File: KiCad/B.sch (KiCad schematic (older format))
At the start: 6 parts

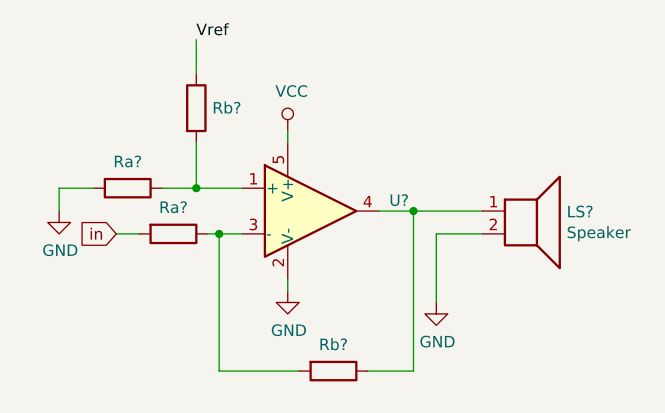
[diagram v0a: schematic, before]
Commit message: update schematics and libraries
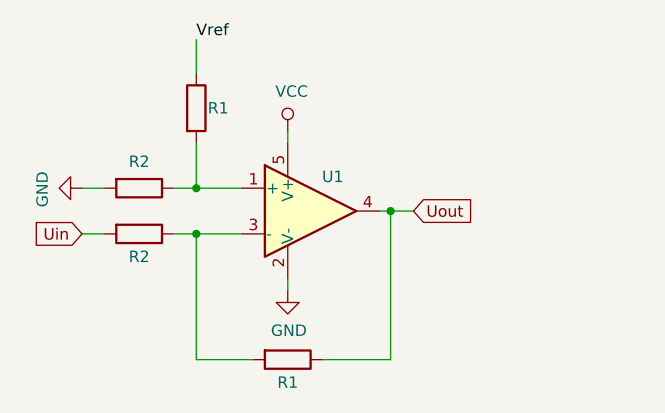
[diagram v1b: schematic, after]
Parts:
- removed LS?: Speaker, symbol Device:Speaker
- Ra3, Ra4: renamed from Ra?; value R -> R2
- Rb3, Rb4: renamed from Rb?; value R -> R1
- U2: renamed from U?; value LM321 -> U1
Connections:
- net Uout: now reaches Rb4.1, U2.4
- net in renamed Uin
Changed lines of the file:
@@
 $EndDescr
 $Comp
-L Amplifier_Operational:LM321 U?
+L Amplifier_Operational:LM321 U2
 U 1 1 617891E9
 P 5750 3750
-F 0 "U?" H 6094 3796 50  0000 L CNN
-F 1 "LM321" H 6094 3705 50  0001 L CNN
+F 0 "U2" H 6094 3796 50  0001 L CNN
+F 1 "U1" H 5800 3900 50  0000 L CNN
 F 2 "Package_TO_SOT_SMD:SOT-23-5" H 5750 3750 50  0001 C CNN
 F 3 "http://www.ti.com/lit/ds/symlink/lm321.pdf" H 5750 3750 50  0001 C CNN
@@
 	1    0    0    -1
 $EndComp
-$Comp
-L Device:Speaker LS?
-U 1 1 617891EF
-P 6700 3750
-F 0 "LS?" H 6870 3746 50  0000 L CNN
-F 1 "Speaker" H 6870 3655 50  0000 L CNN
-F 2 "" H 6700 3550 50  0001 C CNN
-F 3 "~" H 6690 3700 50  0001 C CNN
-	1    6700 3750
-	1    0    0    -1
-$EndComp
 Wire Wire Line
-	6500 3850 6300 3850
-Wire Wire Line
-	6300 3850 6300 4150
-$Comp
-L power:GND #PWR?
-U 1 1 617891F7
-P 6300 4150
-F 0 "#PWR?" H 6300 3900 50  0001 C CNN
-F 1 "GND" H 6305 3977 50  0000 C CNN
-F 2 "" H 6300 4150 50  0001 C CNN
-F 3 "" H 6300 4150 50  0001 C CNN
-	1    6300 4150
-	1    0    0    -1
-$EndComp
-Wire Wire Line
-	5300 3850 5350 3850
+	5150 3850 5250 3850
 Wire Wire Line
 	5450 3650 5250 3650
-Text GLabel 4900 3850 0    50   Input ~ 0
-in
-$Comp
-L Device:R Ra?
-U 1 1 61789200
-P 4950 3650
-F 0 "Ra?" V 4835 3650 50  0000 C CNN
-F 1 "R" V 4834 3650 50  0001 C CNN
-F 2 "" V 4880 3650 50  0001 C CNN
-F 3 "~" H 4950 3650 50  0001 C CNN
-	1    4950 3650
-	0    1    1    0
-$EndComp
-Wire Wire Line
-	4650 3650 4800 3650
+Text GLabel 4750 3850 0    50   Input ~ 0
+Uin
 Wire Wire Line
 	5250 3650 5250 3450
 Connection ~ 5250 3650
 Wire Wire Line
-	5250 3650 5100 3650
+	5250 3650 5150 3650
 $Comp
-L Device:R Rb?
+L Device:R Rb3
 U 1 1 6178920A
 P 5250 3300
-F 0 "Rb?" H 5320 3300 50  0000 L CNN
-F 1 "R" H 5320 3255 50  0001 L CNN
+F 0 "Rb3" H 5320 3300 50  0001 L CNN
+F 1 "R1" H 5300 3300 50  0000 L CNN
 F 2 "" V 5180 3300 50  0001 C CNN
 F 3 "~" H 5250 3300 50  0001 C CNN
@@
 	5650 3450 5650 3400
 $Comp
-L power:VCC #PWR?
+L power:VCC #PWR06
 U 1 1 61789213
 P 5650 3400
-F 0 "#PWR?" H 5650 3250 50  0001 C CNN
+F 0 "#PWR06" H 5650 3250 50  0001 C CNN
 F 1 "VCC" H 5667 3573 50  0000 C CNN
 F 2 "" H 5650 3400 50  0001 C CNN
@@
 	5650 4050 5650 4100
 $Comp
-L power:GND #PWR?
+L power:GND #PWR07
 U 1 1 6178921A
 P 5650 4100
-F 0 "#PWR?" H 5650 3850 50  0001 C CNN
+F 0 "#PWR07" H 5650 3850 50  0001 C CNN
 F 1 "GND" H 5655 3927 50  0000 C CNN
 F 2 "" H 5650 4100 50  0001 C CNN
@@
 	1    0    0    -1
 $EndComp
-Wire Wire Line
-	4650 3650 4650 3750
 $Comp
-L power:GND #PWR?
+L power:GND #PWR05
 U 1 1 61789221
-P 4650 3750
-F 0 "#PWR?" H 4650 3500 50  0001 C CNN
-F 1 "GND" H 4655 3577 50  0000 C CNN
-F 2 "" H 4650 3750 50  0001 C CNN
-F 3 "" H 4650 3750 50  0001 C CNN
-	1    4650 3750
-	1    0    0    -1
-$EndComp
-Wire Wire Line
-	4900 3850 5000 3850
-$Comp
-L Device:R Ra?
-U 1 1 61789228
-P 5150 3850
-F 0 "Ra?" V 5035 3850 50  0000 C CNN
-F 1 "R" V 5034 3850 50  0001 C CNN
-F 2 "" V 5080 3850 50  0001 C CNN
-F 3 "~" H 5150 3850 50  0001 C CNN
-	1    5150 3850
-	0    1    1    0
-$EndComp
-Connection ~ 5350 3850
-Wire Wire Line
-	5350 3850 5450 3850
-Wire Wire Line
-	5350 4450 5700 4450
-Wire Wire Line
-	5350 3850 5350 4450
-$Comp
-L Device:R Rb?
-U 1 1 61789232
-P 5850 4450
-F 0 "Rb?" V 5735 4450 50  0000 C CNN
-F 1 "R" V 5734 4450 50  0001 C CNN
-F 2 "" V 5780 4450 50  0001 C CNN
-F 3 "~" H 5850 4450 50  0001 C CNN
-	1    5850 4450
+P 4750 3650
+F 0 "#PWR05" H 4750 3400 50  0001 C CNN
+F 1 "GND" H 4755 3477 50  0000 C CNN
+F 2 "" H 4750 3650 50  0001 C CNN
+F 3 "" H 4750 3650 50  0001 C CNN
+	1    4750 3650
 	0    1    1    0
 $EndComp
 Wire Wire Line
-	6000 4450 6200 4450
+	4750 3850 4850 3850
+$Comp
+L Device:R Ra4
+U 1 1 61789228
+P 5000 3850
+F 0 "Ra4" V 4885 3850 50  0001 C CNN
+F 1 "R2" V 5100 3850 50  0000 C CNN
+F 2 "" V 4930 3850 50  0001 C CNN
+F 3 "~" H 5000 3850 50  0001 C CNN
+	1    5000 3850
+	0    1    1    0
+$EndComp
+Connection ~ 5250 3850
 Wire Wire Line
-	6200 4450 6200 3750
-Connection ~ 6200 3750
+	5250 3850 5450 3850
 Wire Wire Line
-	6200 3750 6050 3750
+	5250 4400 5500 4400
 Wire Wire Line
-	6200 3750 6500 3750
+	5250 3850 5250 4400
+$Comp
+L Device:R Rb4
+U 1 1 61789232
+P 5650 4400
+F 0 "Rb4" V 5535 4400 50  0001 C CNN
+F 1 "R1" V 5750 4400 50  0000 C CNN
+F 2 "" V 5580 4400 50  0001 C CNN
+F 3 "~" H 5650 4400 50  0001 C CNN
+	1    5650 4400
+	0    1    1    0
+$EndComp
+Wire Wire Line
+	5800 4400 6100 4400
+Wire Wire Line
+	6100 4400 6100 3750
+Connection ~ 6100 3750
+Wire Wire Line
+	6100 3750 6050 3750
+Wire Wire Line
+	6100 3750 6200 3750
+$Comp
+L Device:R Ra3
+U 1 1 61789200
+P 5000 3650
+F 0 "Ra3" V 4885 3650 50  0001 C CNN
+F 1 "R2" V 4884 3650 50  0000 C CNN
+F 2 "" V 4930 3650 50  0001 C CNN
+F 3 "~" H 5000 3650 50  0001 C CNN
+	1    5000 3650
+	0    1    1    0
+$EndComp
+Wire Wire Line
+	4750 3650 4850 3650
+Text GLabel 6200 3750 2    50   Input ~ 0
+Uout
 $EndSCHEMATC
